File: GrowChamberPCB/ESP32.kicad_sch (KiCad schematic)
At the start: 29 parts, among them SW1 Reset_Button_Internal, SW3 Bootmode_Internal, U3 ESP32-S3-WROOM-1U-N8R8, U7 TC4428EOA, U8 W25Q128JVSIQTR

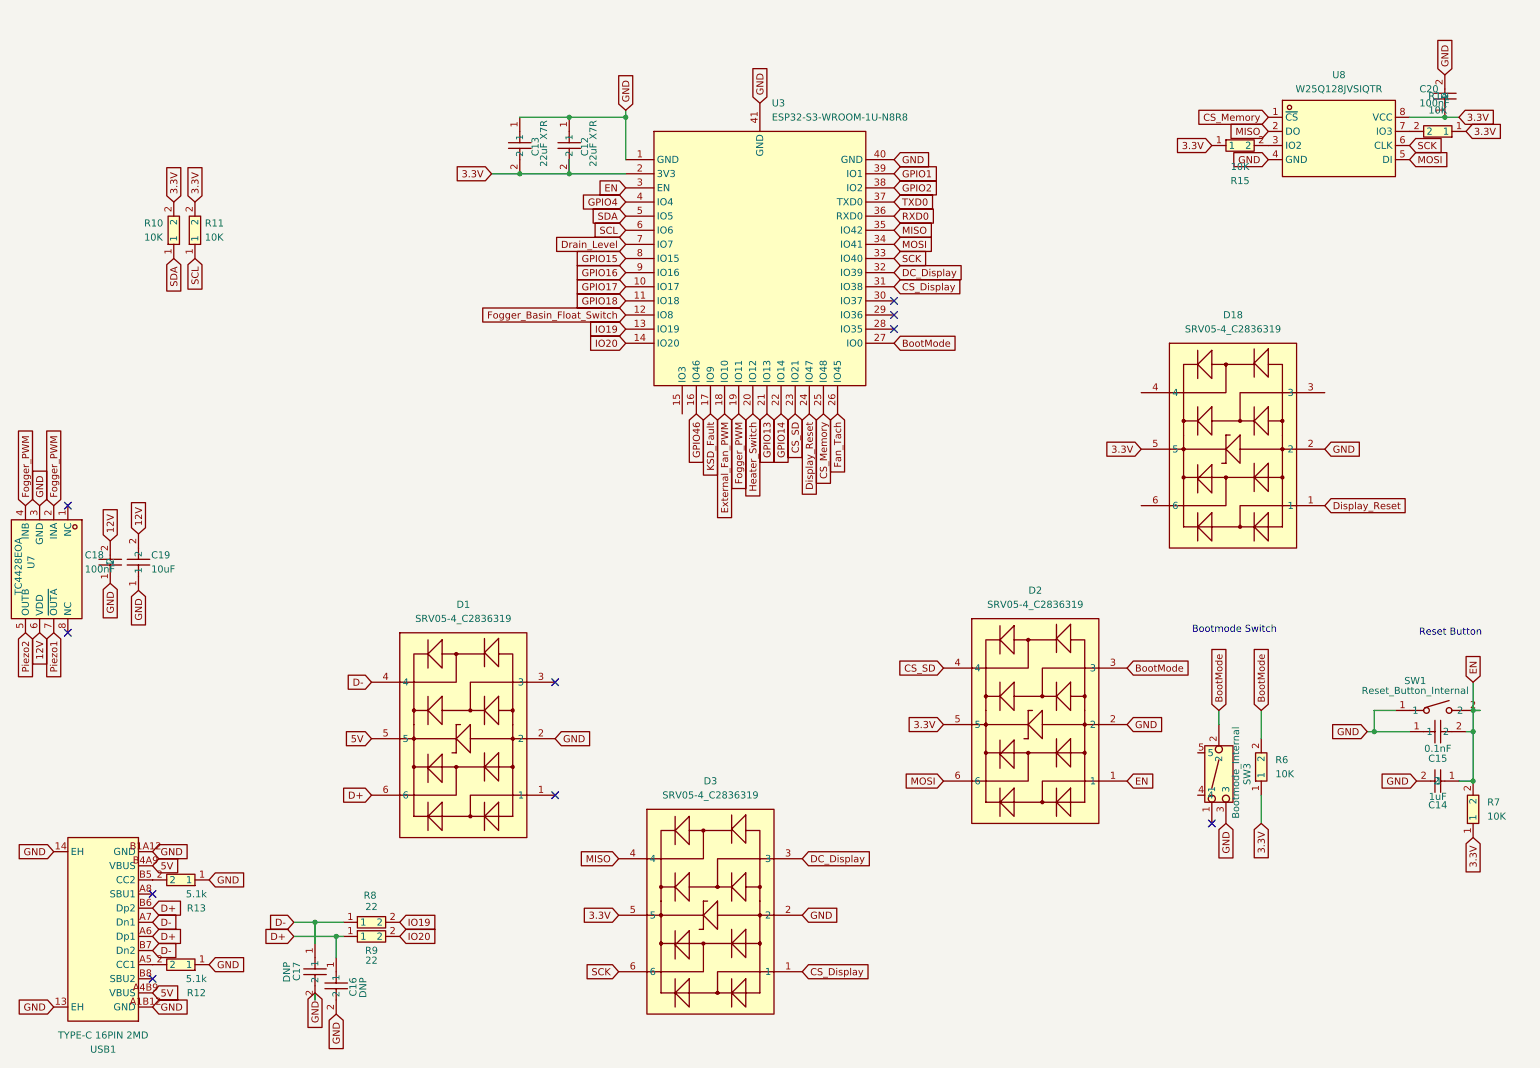
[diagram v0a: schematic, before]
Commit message: almost done!
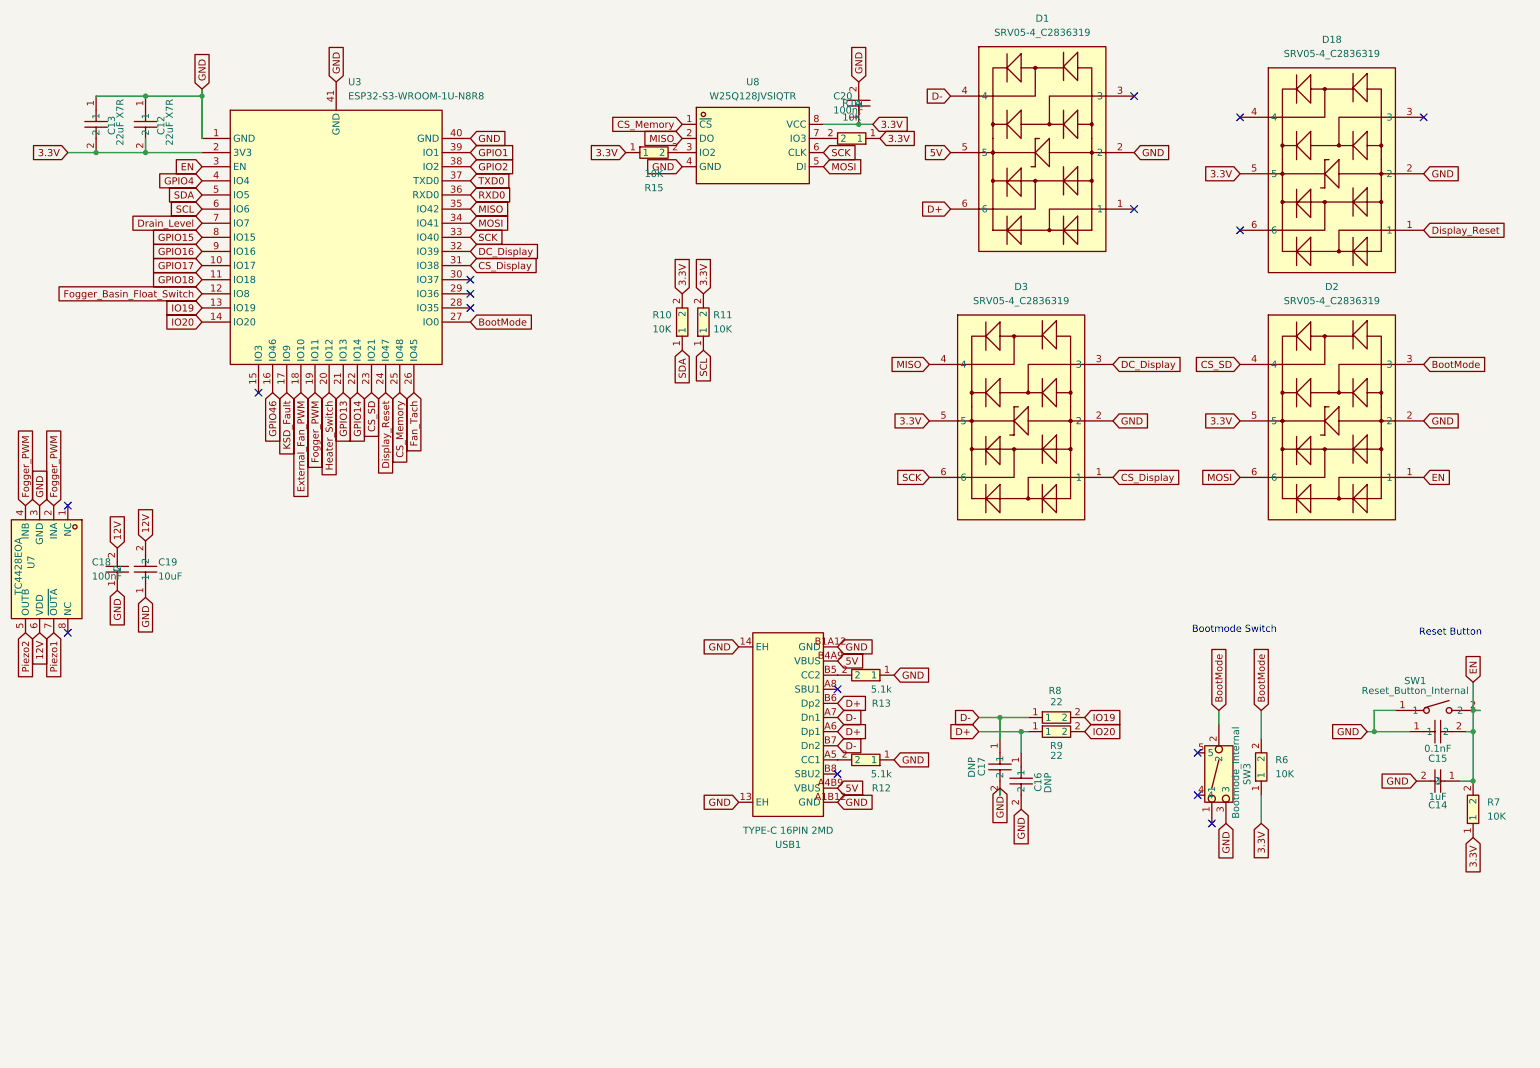
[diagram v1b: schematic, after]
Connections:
- no-connect marks 10 -> 16
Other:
- moved on the sheet: C12, C13, C16, C17, C18, C19, C20, D1, D18, D2, D3, R10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
